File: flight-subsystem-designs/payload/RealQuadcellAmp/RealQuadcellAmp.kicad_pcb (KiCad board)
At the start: 2 copper layers, 109.8 x 90.5 mm, 92 parts, among them J1 Screw_Terminal_01x02, J2 Conn_01x04_Pin, J3 Conn_01x04_Pin, U1 LM2904, U2 LM2904, U3 LM2904, U4 LM2904, U6 L78L33_SOT89, U6 LM2904

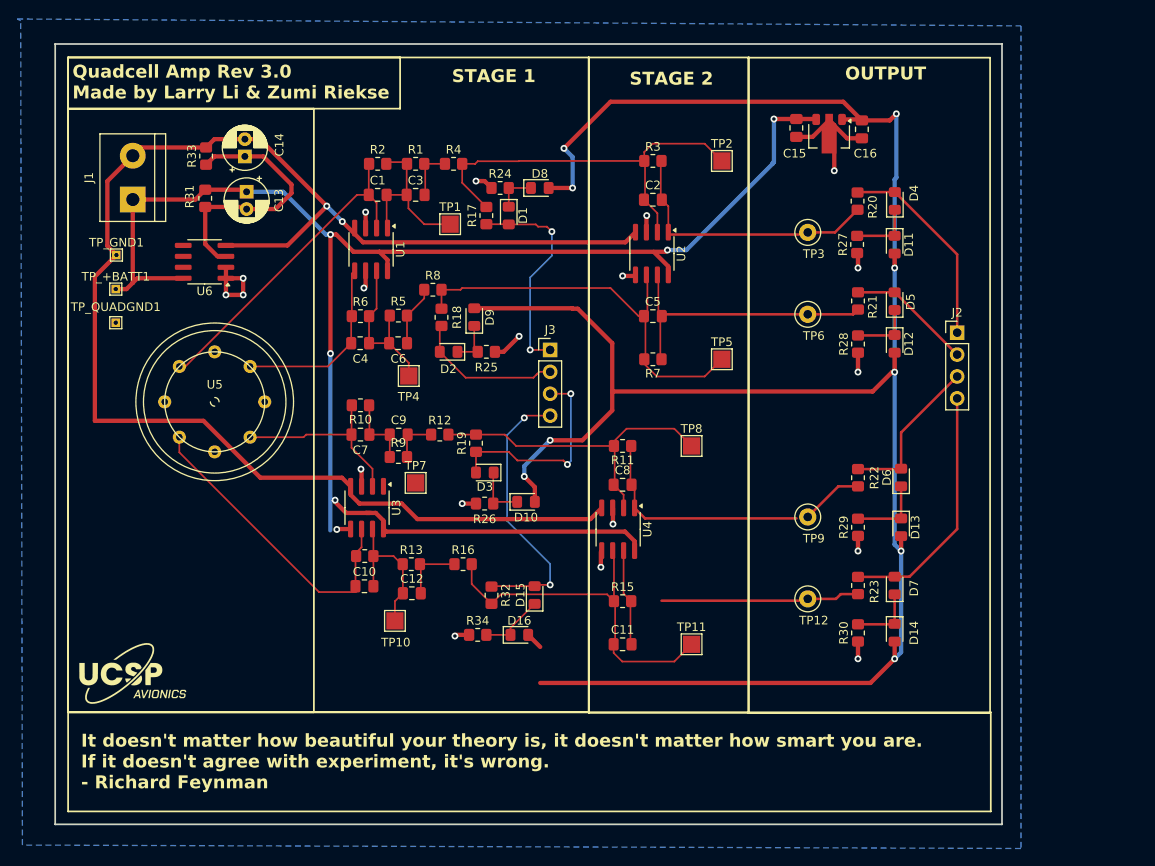
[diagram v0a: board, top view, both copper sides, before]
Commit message: fix: connected stage2
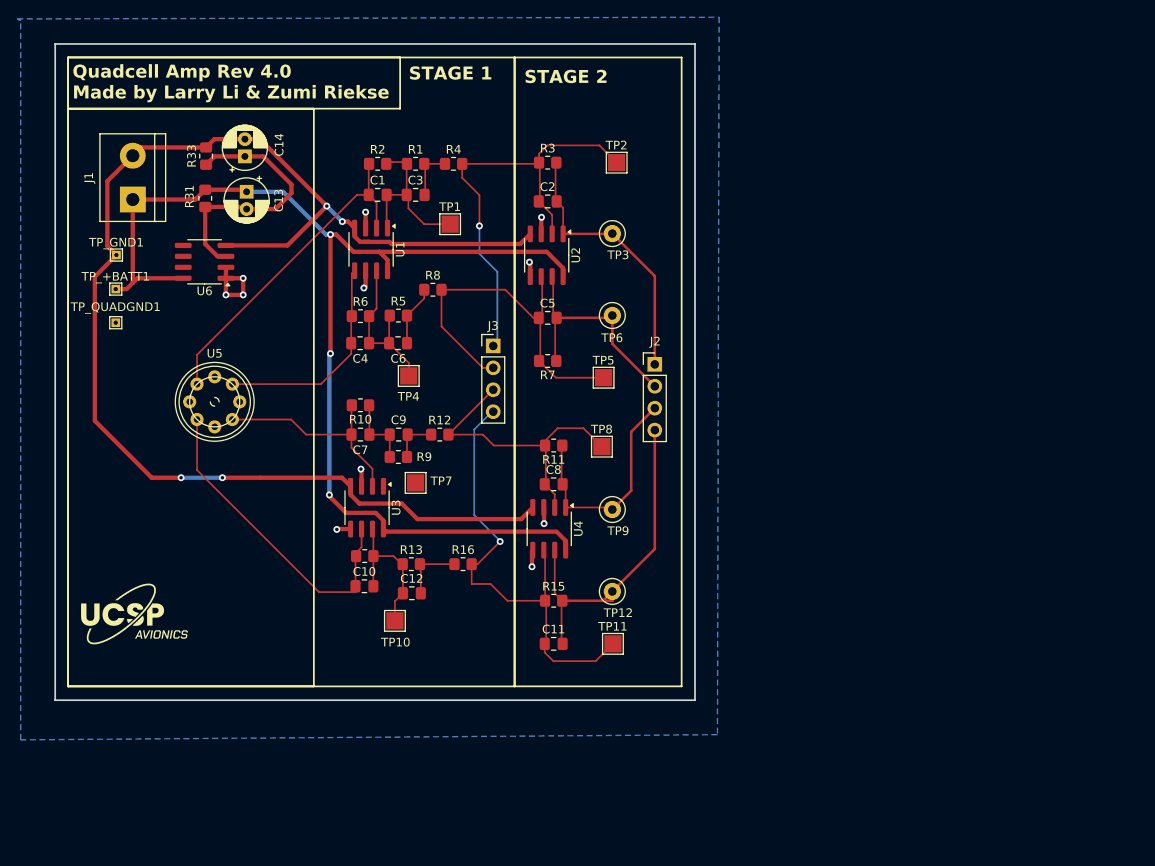
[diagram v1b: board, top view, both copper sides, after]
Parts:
- removed C15: 0.33u, Capacitor_SMD:C_0805_2012Metric_Pad1.18x1.45mm_HandSolder
- removed C16: 0.1u, Capacitor_SMD:C_0805_2012Metric_Pad1.18x1.45mm_HandSolder
- removed D1, D10, D11, D12, D13, D14, D15, D16, D2, D3, D4, D5, D6, D7, D8, D9: ~, Diode_SMD:D_0805_2012Metric_Pad1.15x1.40mm_HandSolder
- removed R17, R18, R19, R20, R21, R22, R23, R32: 1 kΩ, Resistor_SMD:R_0805_2012Metric_Pad1.20x1.40mm_HandSolder
- removed R24, R25, R26, R27, R28, R29, R30, R34: 40 Ω, Resistor_SMD:R_0805_2012Metric_Pad1.20x1.40mm_HandSolder
- removed the U6 at (173.8, 50.2)
- moved J2 35.3 mm to (153.5, 76.7)
- moved TP12 22.7 mm to (148.6, 103.0)
- moved TP9 22.7 mm to (148.6, 93.5)
- moved TP3 22.7 mm to (148.6, 61.5)
- moved TP6 22.7 mm to (148.6, 71.0)
- moved TP5 13.9 mm to (147.6, 78.2)
- moved C2 12.2 mm to (141.1, 57.8)
- moved C5 12.2 mm to (141.1, 71.3)
- moved R3 12.2 mm to (141.1, 53.3)
- moved R7 12.2 mm to (141.1, 76.3)
- moved TP2 12.2 mm to (149.1, 53.3)
- moved U2 12.2 mm to (141.0, 64.0)
- moved TP8 10.4 mm to (147.4, 86.2)
- moved TP11 9.12 mm to (148.7, 109.1)
- moved C11 7.99 mm to (141.8, 109.1)
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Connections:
- J2 pad 1: /FOUT1 -> /STAGE2_OUT1
- J2 pad 2: /FOUT2 -> /STAGE2_OUT2
- J2 pad 3: /FOUT3 -> /STAGE2_OUT3
- J2 pad 4: /FOUT4 -> /STAGE2_OUT4
- J3 pad 1: /MOUT1 -> /STAGE1_OUT1
- J3 pad 2: /MOUT2 -> /STAGE1_OUT2
- J3 pad 3: /MOUT3 -> /STAGE1_OUT3
- J3 pad 4: /MOUT4 -> /STAGE1_OUT4
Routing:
- net +3V3: track 244.6 -> 0.00 mm, vias 9 -> 0
- net VCC: track 189.6 -> 137.4 mm, vias 5 -> 3
- net /MOUT4: track 32.3 -> 0.00 mm, vias 2 -> 0
- net QUAD_GND: track 56.3 -> 24.0 mm, vias 20 -> 11
- net /FOUT4: track 28.9 -> 0.00 mm
- net /MOUT1: track 25.0 -> 0.00 mm, vias 2 -> 0
- net /MOUT3: track 24.7 -> 0.00 mm, vias 2 -> 0
- net /FOUT1: track 23.6 -> 0.00 mm
- net GND: track 176.2 -> 157.3 mm, vias 2 -> 4
- net /FOUT3: track 18.4 -> 0.00 mm
- net /MOUT2: track 17.4 -> 0.00 mm
- net /FOUT2: track 14.5 -> 0.00 mm
- net /STAGE1_OUT4: track 43.3 -> 54.7 mm, vias 0 -> 1
- net Net-(D13-K): track 8.74 -> 0.00 mm
- net Net-(D14-K): track 7.70 -> 0.00 mm
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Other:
- board size 109.8 x 90.5 mm -> 74.2 x 76.1 mm
- board text added: "Quadcell Amp Rev 4.0 Made by Larry Li & Zumi Riekse"
- board text removed: "It doesn't matter how beautiful your theory is, it doesn't matter how smart you are. If it doesn't agree with experiment, it's wrong. - Richard Feynman"
- board text removed: "OUTPUT"
- board text removed: "Quadcell Amp Rev 3.0 Made by Larry Li & Zumi Riekse"
